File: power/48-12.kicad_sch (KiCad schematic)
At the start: 13 parts, among them U1 BMR4800116/005, U2 HO150-NP

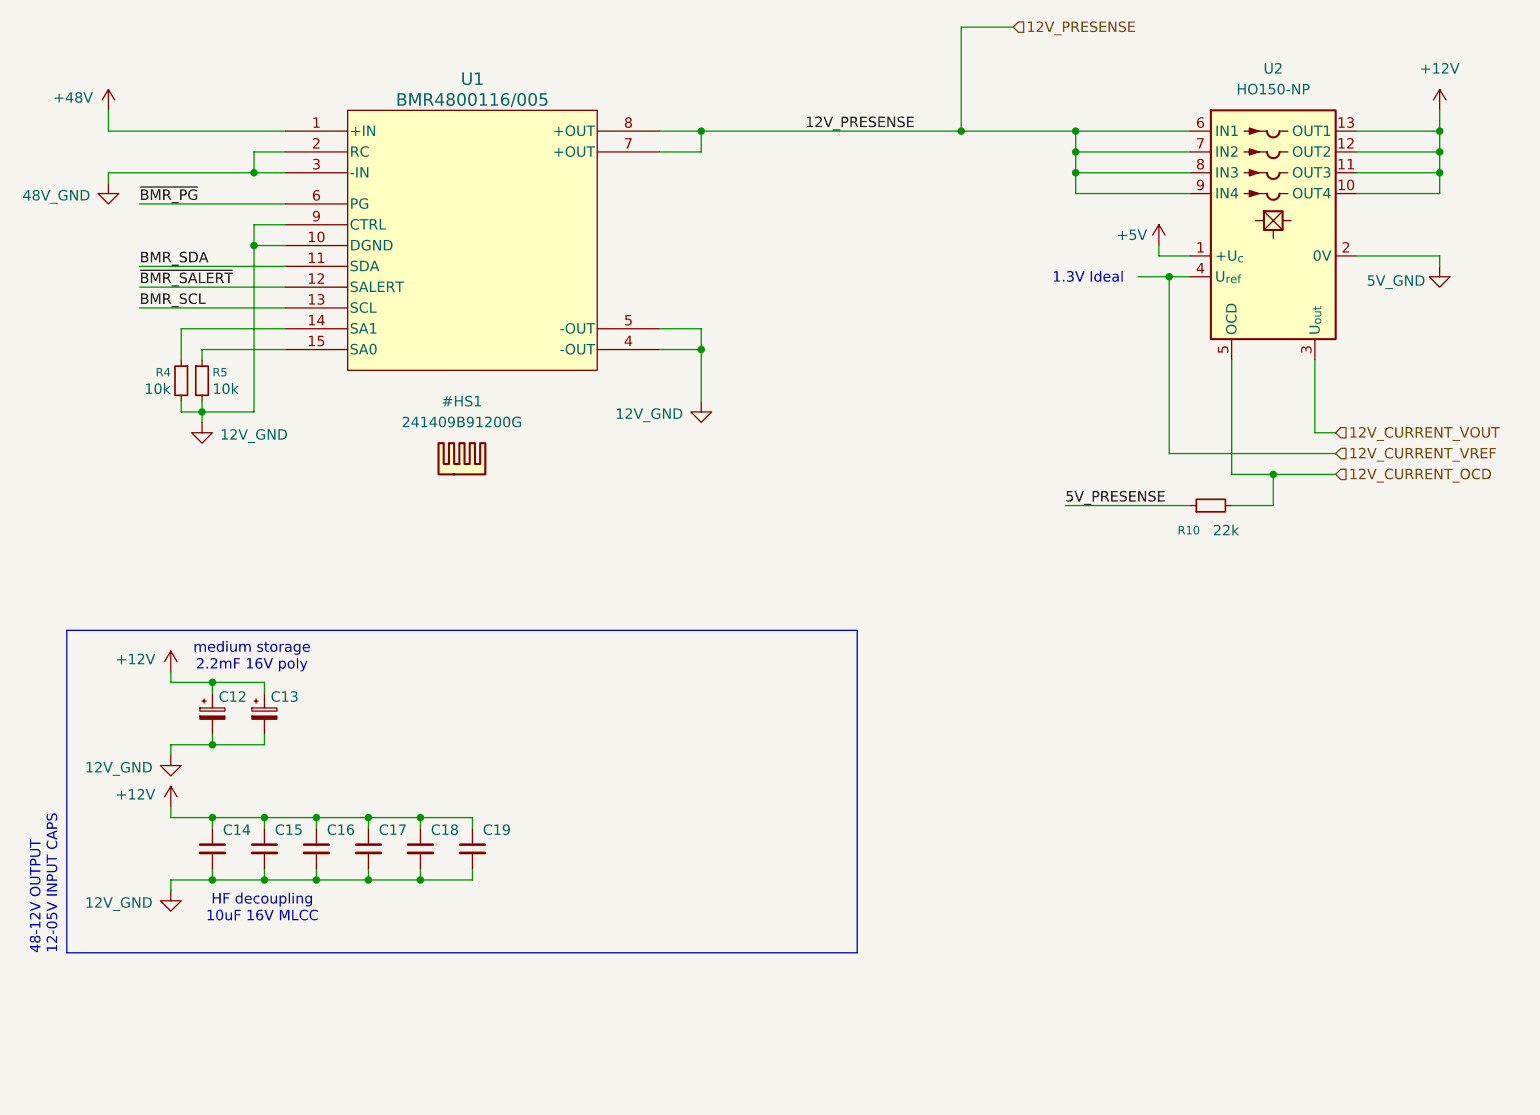
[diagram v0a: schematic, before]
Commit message: work
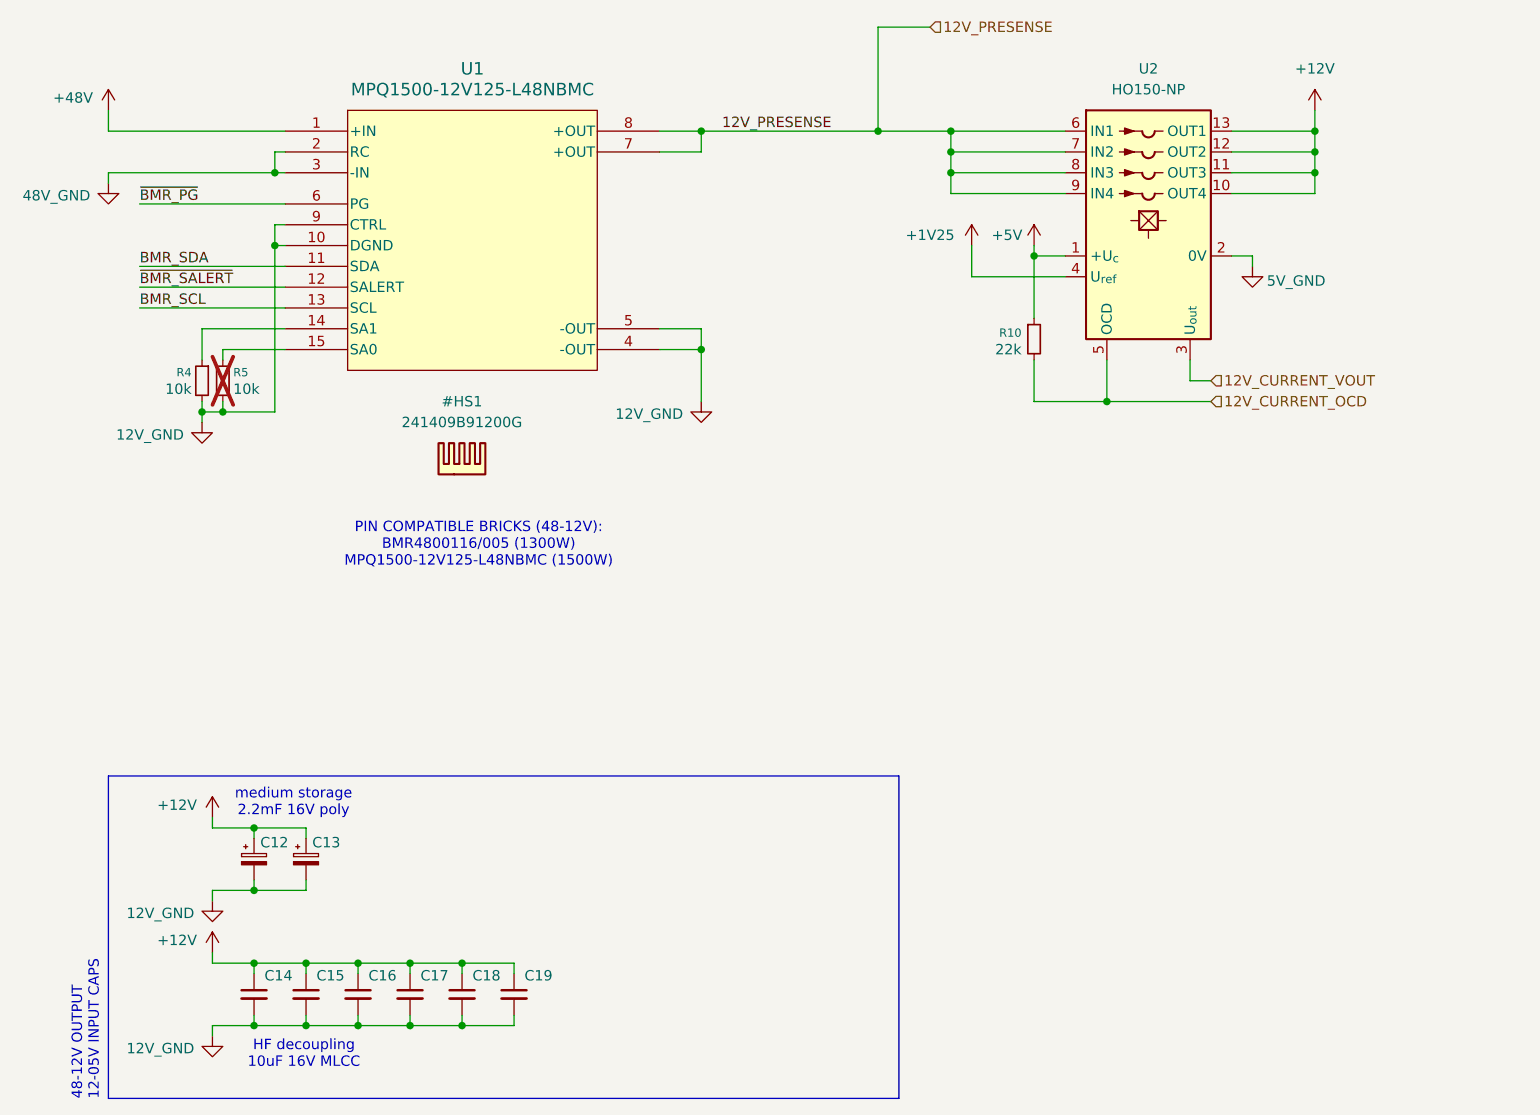
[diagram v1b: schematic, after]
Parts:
- R5: now not fitted
- U1: value BMR4800116/005 -> MPQ1500-12V125-L48NBMC
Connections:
- net 5V_PRESENSE is gone; now on net +5V: R10.1
- net 12V_CURRENT_VREF renamed +1V25
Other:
- note added: "PIN COMPATIBLE BRICKS (48-12V): BMR4800116/005 (1300W) MPQ1500-12V125-L48NBMC (1500W)"
- note removed: "1.3V Ideal"
- moved on the sheet: C12, C13, C14, C15, C16, C17, C18, C19, R10, R4, U2
